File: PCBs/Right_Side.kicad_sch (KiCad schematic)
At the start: 76 parts, among them J4 USB_C_Receptacle, J6 USB_C_Receptacle, U5 W25Q128JVS, U6 XC6206-3.3_SOT, U7 USBLC6-2SC6, U8 RP2040, Y2 Crystal_GND24

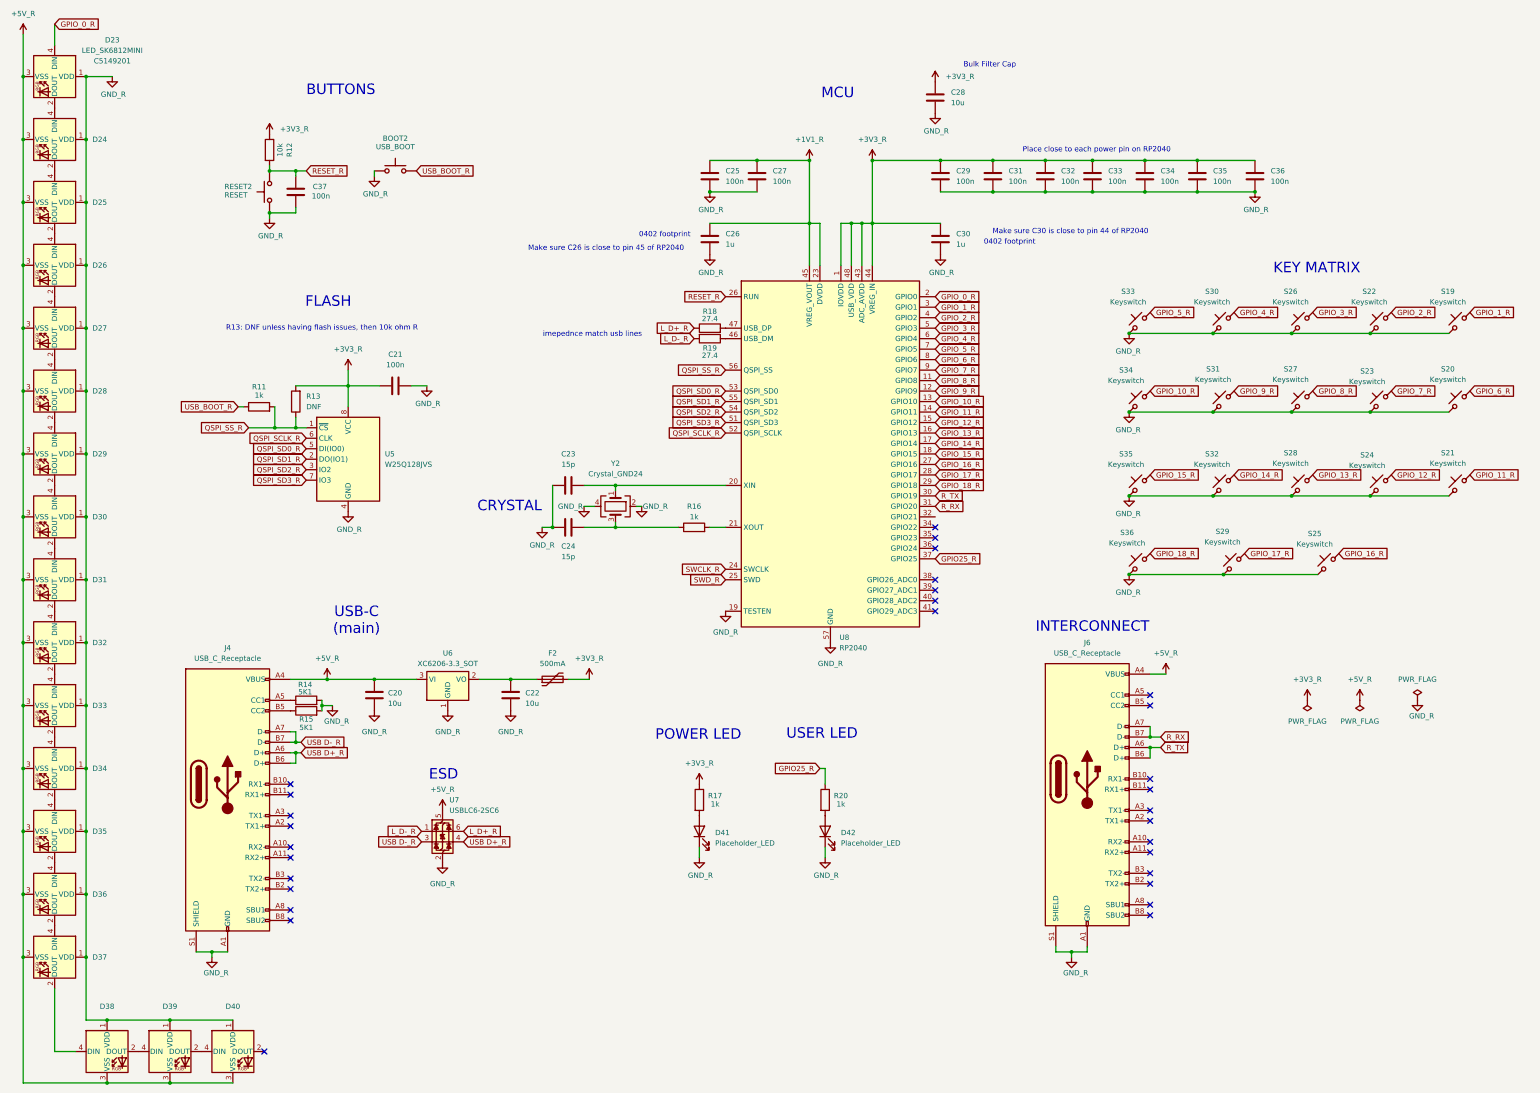
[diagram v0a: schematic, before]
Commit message: mid way right side
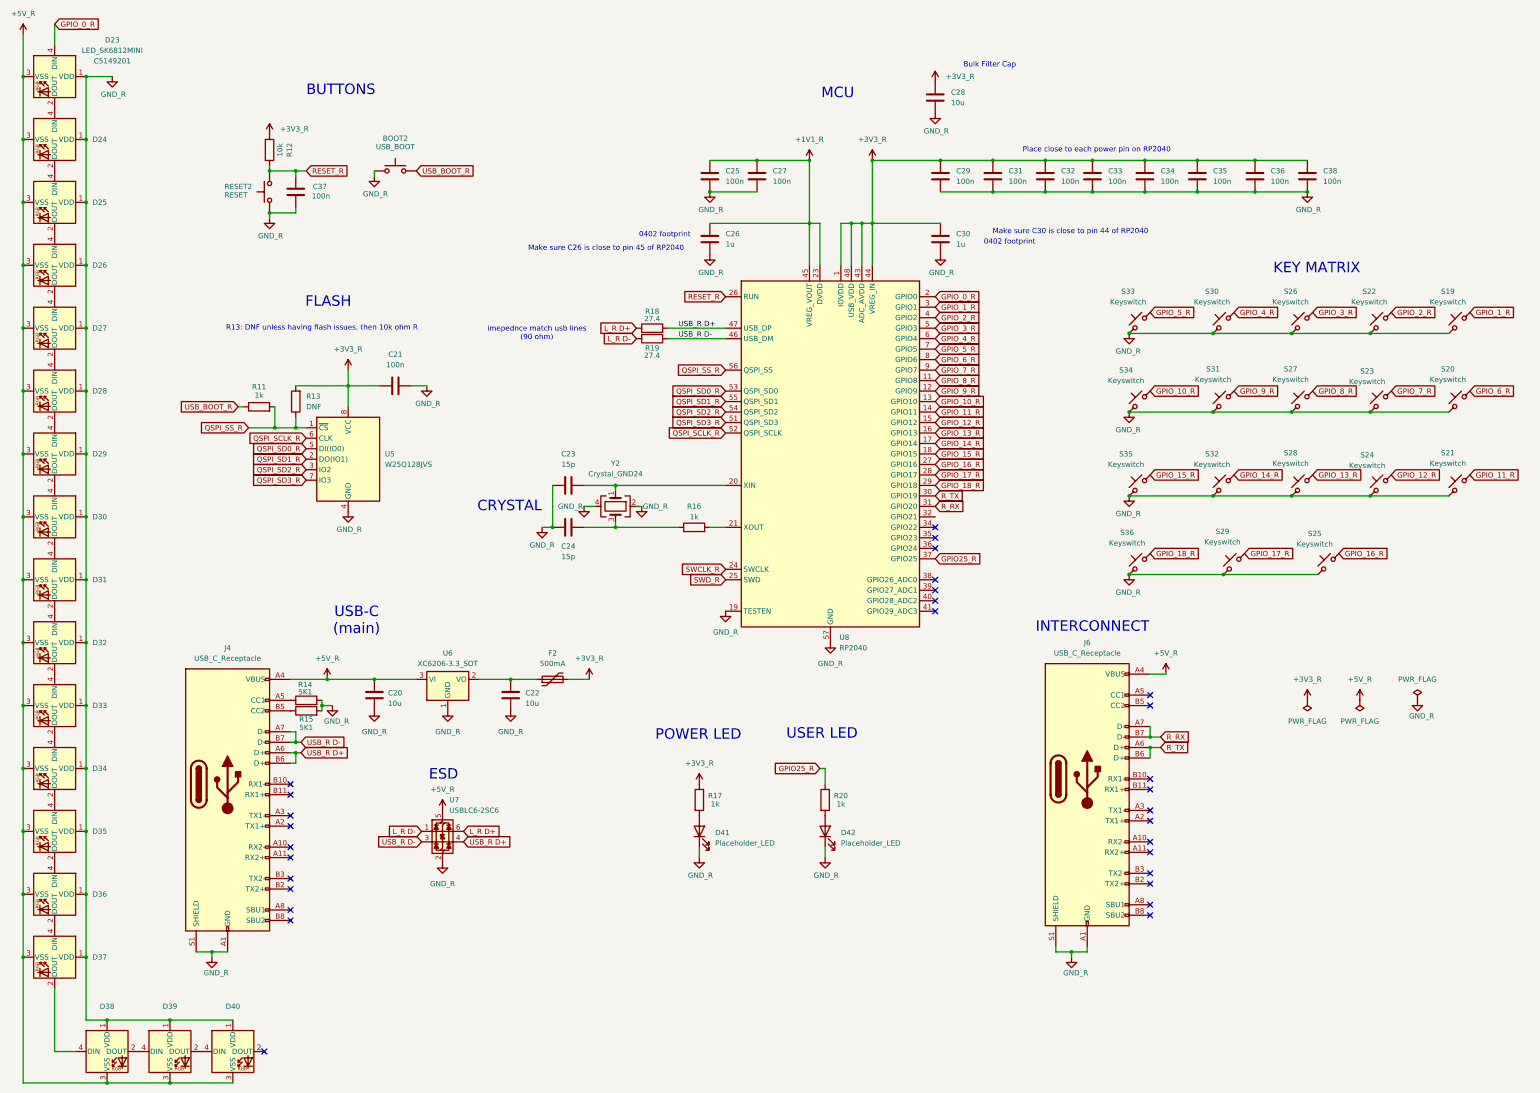
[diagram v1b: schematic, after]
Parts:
- added C38: 100n, Capacitor_SMD:C_0603_1608Metric, symbol Device:C
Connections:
- net USB D+_R is gone; now on net USB_R D+: J4.A6 (D+), J4.B6 (D+), U7.4 (I/O2)
- net USB D-_R is gone; now on net USB_R D-: J4.A7 (D-), J4.B7 (D-), U7.3 (I/O2)
- net +3V3_R: now also C38.1
- net GND_R: now also C38.2
- net USB_R D-: now reaches R19.1, U8.46 (USB_DM)
- net USB_R D+: now reaches R18.2, U8.47 (USB_DP)
- net L_D+_R renamed L_R D+
- net L_D-_R renamed L_R D-
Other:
- note added: "imepednce match usb lines (90 ohm)"
- note removed: "imepednce match usb lines"
- moved on the sheet: R18, R19
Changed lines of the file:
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@@
 	)
 	(junction
+		(at 322.58 54.61)
+		(diameter 0)
+		(color 0 0 0 0)
+	)
+	(junction
+		(at 335.28 62.23)
+		(diameter 0)
+		(color 0 0 0 0)
+	)
+	(junction
 		(at 292.1 115.57)
 		(diameter 0)
@@
 	(wire
 		(pts
+			(xy 180.34 95.25) (xy 194.31 95.25)
+		)
+		(stroke
+			(width 0)
+			(type default)
+		)
+	)
+	(wire
+		(pts
 			(xy 331.47 135.89) (xy 312.42 135.89)
 		)
@@
 	(wire
 		(pts
-			(xy 229.87 69.85) (xy 229.87 80.01)
+			(xy 335.28 62.23) (xy 322.58 62.23)
 		)
 		(stroke
@@
 	(wire
 		(pts
-			(xy 90.17 109.22) (xy 102.87 109.22)
+			(xy 229.87 69.85) (xy 229.87 80.01)
 		)
 		(stroke
@@
 	(wire
 		(pts
-			(xy 24.13 80.01) (xy 24.13 95.25)
+			(xy 90.17 109.22) (xy 102.87 109.22)
 		)
 		(stroke
@@
 	(wire
 		(pts
-			(xy 85.09 119.38) (xy 90.17 119.38)
+			(xy 24.13 80.01) (xy 24.13 95.25)
 		)
 		(stroke
@@
 	(wire
 		(pts
-			(xy 322.58 54.61) (xy 308.61 54.61)
+			(xy 85.09 119.38) (xy 90.17 119.38)
 		)
 		(stroke
@@
 	(wire
 		(pts
+			(xy 180.34 97.79) (xy 194.31 97.79)
+		)
+		(stroke
+			(width 0)
+			(type default)
+		)
+	)
+	(wire
+		(pts
 			(xy 69.85 246.38) (xy 73.66 246.38)
 		)
@@
 	(wire
 		(pts
+			(xy 308.61 54.61) (xy 322.58 54.61)
+		)
+		(stroke
+			(width 0)
+			(type default)
+		)
+	)
+	(wire
+		(pts
 			(xy 24.13 201.93) (xy 24.13 217.17)
 		)
@@
 	(wire
 		(pts
+			(xy 335.28 54.61) (xy 322.58 54.61)
+		)
+		(stroke
+			(width 0)
+			(type default)
+		)
+	)
+	(wire
+		(pts
 			(xy 312.42 135.89) (xy 292.1 135.89)
 		)
@@
 		)
 	)
-	(text "imepednce match usb lines\n"
+	(text "imepednce match usb lines\n(90 ohm)\n"
 		(exclude_from_sim no)
-		(at 162.052 96.774 0)
+		(at 148.59 96.52 0)
 		(effects
 			(font
@@
 		)
 	)
-	(global_label "USB D-_R"
+	(label "USB_R D+"
+		(at 182.88 95.25 0)
+		(effects
+			(font
+				(size 1.27 1.27)
+			)
+			(justify left bottom)
+		)
+	)
+	(label "USB_R D-"
+		(at 182.88 97.79 0)
+		(effects
+			(font
+				(size 1.27 1.27)
+			)
+			(justify left bottom)
+		)
+	)
+	(global_label "USB_R D-"
 		(shape input)
 		(at 120.65 219.71 180)
@@
 		)
 	)
-	(global_label "L_D+_R"
+	(global_label "L_R D+"
 		(shape input)
-		(at 186.69 95.25 180)
+		(at 172.72 95.25 180)
 		(fields_autoplaced yes)
 		(effects
@@
 		)
 		(property "Intersheetrefs" "${INTERSHEET_REFS}"
-			(at 176.6291 95.25 0)
+			(at 162.6591 95.25 0)
 			(effects
 				(font
@@
 		)
 	)
-	(global_label "L_D-_R"
+	(global_label "L_R D-"
 		(shape input)
 		(at 120.65 217.17 180)
@@
 		)
 	)
-	(global_label "L_D+_R"
+	(global_label "L_R D+"
 		(shape input)
 		(at 130.81 217.17 0)
@@
 		)
 	)
-	(global_label "L_D-_R"
+	(global_label "L_R D-"
 		(shape input)
-		(at 186.69 97.79 180)
+		(at 172.72 97.79 180)
 		(fields_autoplaced yes)
 		(effects
@@
 		)
 		(property "Intersheetrefs" "${INTERSHEET_REFS}"
-			(at 176.6291 97.79 0)
+			(at 162.6591 97.79 0)
 			(effects
 				(font
@@
 		)
 	)
-	(global_label "USB D-_R"
+	(global_label "USB_R D-"
 		(shape input)
 		(at 91.44 195.58 0)
@@
 		)
 	)
-	(global_label "USB D+_R"
+	(global_label "USB_R D+"
 		(shape input)
 		(at 130.81 219.71 0)
@@
 		)
 	)
-	(global_label "USB D+_R"
+	(global_label "USB_R D+"
 		(shape input)
 		(at 91.44 198.12 0)
@@
 	(symbol
 		(lib_id "Device:R")
-		(at 190.5 97.79 270)
+		(at 176.53 97.79 270)
 		(unit 1)
 		(exclude_from_sim no)
@@
 		(dnp no)
 		(property "Reference" "R19"
-			(at 190.5 100.076 90)
+			(at 176.53 100.076 90)
 			(effects
 				(font
@@
 		)
 		(property "Value" "27.4"
-			(at 190.5 101.854 90)
+			(at 176.53 101.854 90)
 			(effects
 				(font
@@
 		)
 		(property "Footprint" "Resistor_SMD:R_0603_1608Metric"
-			(at 190.5 96.012 90)
+			(at 176.53 96.012 90)
 			(effects
 				(font
@@
 		)
 		(property "Datasheet" "~"
-			(at 190.5 97.79 0)
+			(at 176.53 97.79 0)
 			(effects
 				(font
@@
 		)
 		(property "Description" "Resistor"
-			(at 190.5 97.79 0)
+			(at 176.53 97.79 0)
 			(effects
 				(font
@@
 	)
 	(symbol
+		(lib_id "Device:C")
+		(at 335.28 58.42 0)
+		(unit 1)
+		(exclude_from_sim no)
+		(in_bom yes)
+		(on_board yes)
+		(dnp no)
+		(fields_autoplaced yes)
+		(property "Reference" "C38"
+			(at 339.09 57.1499 0)
+			(effects
+				(font
+					(size 1.27 1.27)
+				)
+				(justify left)
+			)
+		)
+		(property "Value" "100n"
+			(at 339.09 59.6899 0)
+			(effects
+				(font
+					(size 1.27 1.27)
+				)
+				(justify left)
+			)
+		)
+		(property "Footprint" "Capacitor_SMD:C_0603_1608Metric"
+			(at 336.2452 62.23 0)
+			(effects
+				(font
+					(size 1.27 1.27)
+				)
+				(hide yes)
+			)
+		)
+		(property "Datasheet" "~"
+			(at 335.28 58.42 0)
+			(effects
+				(font
+					(size 1.27 1.27)
+				)
+				(hide yes)
+			)
+		)
+		(property "Description" "Unpolarized capacitor"
+			(at 335.28 58.42 0)
+			(effects
+				(font
+					(size 1.27 1.27)
+				)
+				(hide yes)
+			)
+		)
+		(pin "1"
+		)
+		(pin "2"
+		)
+		(instances
+			(project "CustomKB2040"
+				(path "/1dc59942-63a2-41f5-a9fb-7502b7672a2f/509c21e9-3c87-4ca7-a30c-cd35896bf815"
+					(reference "C38")
+					(unit 1)
+				)
+			)
+		)
+	)
+	(symbol
 		(lib_id "ScottoKeebs:LED_SK6812MINI")
 		(at 31.75 110.49 270)
@@
 	(symbol
 		(lib_id "power:GND")
-		(at 322.58 62.23 0)
+		(at 335.28 62.23 0)
 		(unit 1)
 		(exclude_from_sim no)
@@
 		(dnp no)
 		(property "Reference" "#PWR075"
-			(at 322.58 68.58 0)
+			(at 335.28 68.58 0)
 			(effects
 				(font
@@
 		)
 		(property "Value" "GND_R"
-			(at 322.834 66.548 0)
+			(at 335.534 66.548 0)
 			(effects
 				(font
@@
 		)
 		(property "Footprint" ""
-			(at 322.58 62.23 0)
+			(at 335.28 62.23 0)
 			(effects
 				(font
@@
 		)
 		(property "Datasheet" ""
-			(at 322.58 62.23 0)
+			(at 335.28 62.23 0)
 			(effects
 				(font
@@
 		)
 		(property "Description" "Power symbol creates a global label with name \"GND\" , ground"
-			(at 322.58 62.23 0)
+			(at 335.28 62.23 0)
 			(effects
 				(font
@@
 	(symbol
 		(lib_id "Device:R")
-		(at 190.5 95.25 90)
+		(at 176.53 95.25 90)
 		(unit 1)
 		(exclude_from_sim no)
@@
 		(dnp no)
 		(property "Reference" "R18"
-			(at 190.5 91.186 90)
+			(at 176.53 91.186 90)
 			(effects
 				(font
@@
 		)
 		(property "Value" "27.4"
-			(at 190.5 92.964 90)
+			(at 176.53 92.964 90)
 			(effects
 				(font
@@
 		)
 		(property "Footprint" "Resistor_SMD:R_0603_1608Metric"
-			(at 190.5 97.028 90)
+			(at 176.53 97.028 90)
 			(effects
 				(font
@@
 		)
 		(property "Datasheet" "~"
-			(at 190.5 95.25 0)
+			(at 176.53 95.25 0)
 			(effects
 				(font
@@
 		)
 		(property "Description" "Resistor"
-			(at 190.5 95.25 0)
+			(at 176.53 95.25 0)
 			(effects
 				(font

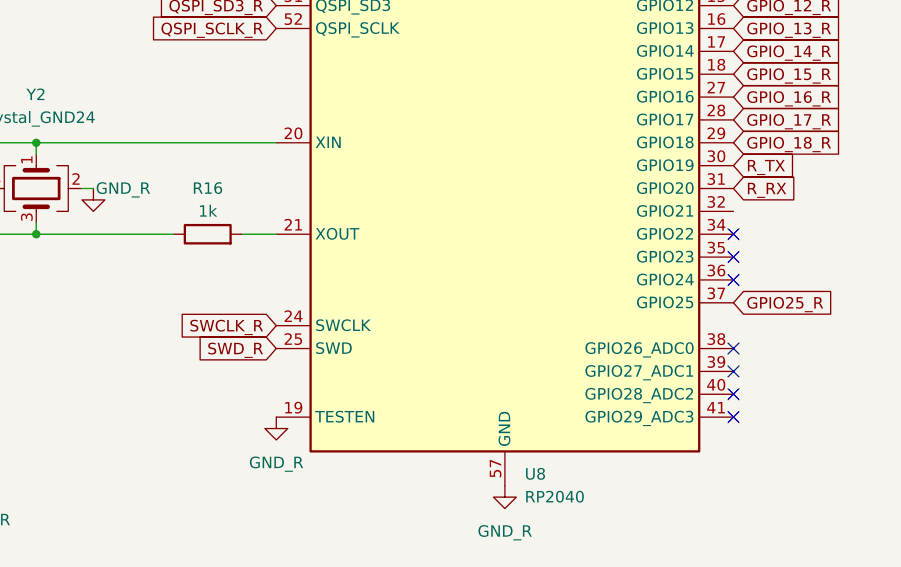
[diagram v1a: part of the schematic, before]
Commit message: making progress
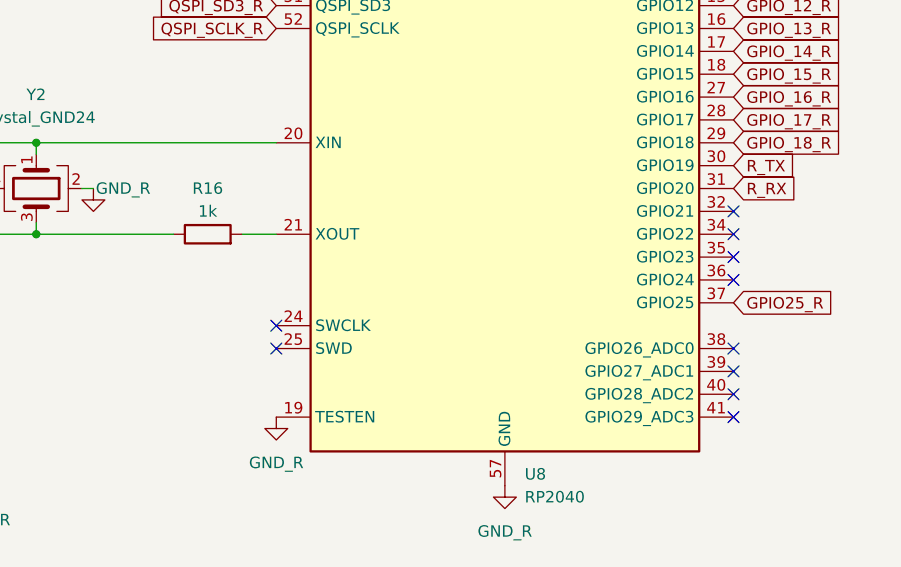
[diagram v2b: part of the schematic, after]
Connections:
- net SWCLK_R: no longer names the net of U8.24 (SWCLK)
- net SWD_R: no longer names the net of U8.25 (SWD)
- no-connect marks 30 -> 33
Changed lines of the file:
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@@
+	)
+	(no_connect
+		(at 194.31 156.21)
 	)
 	(no_connect
@@
 	)
 	(no_connect
+		(at 245.11 140.97)
+	)
+	(no_connect
 		(at 88.9 223.52)
 	)
@@
 	(no_connect
 		(at 88.9 231.14)
+	)
+	(no_connect
+		(at 194.31 153.67)
 	)
 	(no_connect
@@
 		)
 	)
-	(global_label "SWD_R"
-		(shape input)
-		(at 194.31 156.21 180)
+	(global_label "QSPI_SD1_R"
+		(shape input)
+		(at 194.31 113.03 180)
 		(fields_autoplaced yes)
 		(effects
@@
 		)
 		(property "Intersheetrefs" "${INTERSHEET_REFS}"
-			(at 185.1563 156.21 0)
+			(at 180.0158 113.03 0)
 			(effects
 				(font
@@
 		)
 	)
-	(global_label "QSPI_SD1_R"
-		(shape input)
-		(at 194.31 113.03 180)
+	(global_label "GPIO_4_R"
+		(shape input)
+		(at 317.5 91.44 0)
+		(fields_autoplaced yes)
+		(effects
+			(font
+				(size 1.27 1.27)
+			)
+			(justify left)
+		)
+		(property "Intersheetrefs" "${INTERSHEET_REFS}"
+			(at 329.3752 91.44 0)
+			(effects
+				(font
+					(size 1.27 1.27)
+				)
+				(justify left)
+				(hide yes)
+			)
+		)
+	)
+	(global_label "QSPI_SD2_R"
+		(shape input)
+		(at 92.71 129.54 180)
 		(fields_autoplaced yes)
 		(effects
@@
 		)
 		(property "Intersheetrefs" "${INTERSHEET_REFS}"
-			(at 180.0158 113.03 0)
+			(at 78.4158 129.54 0)
 			(effects
 				(font
@@
 		)
 	)
-	(global_label "GPIO_4_R"
-		(shape input)
-		(at 317.5 91.44 0)
-		(fields_autoplaced yes)
-		(effects
-			(font
-				(size 1.27 1.27)
-			)
-			(justify left)
-		)
-		(property "Intersheetrefs" "${INTERSHEET_REFS}"
-			(at 329.3752 91.44 0)
-			(effects
-				(font
-					(size 1.27 1.27)
-				)
-				(justify left)
-				(hide yes)
-			)
-		)
-	)
-	(global_label "QSPI_SD2_R"
-		(shape input)
-		(at 92.71 129.54 180)
-		(fields_autoplaced yes)
-		(effects
-			(font
-				(size 1.27 1.27)
-			)
-			(justify right)
-		)
-		(property "Intersheetrefs" "${INTERSHEET_REFS}"
-			(at 78.4158 129.54 0)
-			(effects
-				(font
-					(size 1.27 1.27)
-				)
-				(justify right)
-				(hide yes)
-			)
-		)
-	)
 	(global_label "USB_R D+"
 		(shape input)
@@
 				(hide yes)
 			)
-		)
-	)
-	(global_label "SWCLK_R"
-		(shape input)
-		(at 194.31 153.67 180)
-		(fields_autoplaced yes)
-		(effects
-			(font
-				(size 1.27 1.27)
-			)
-			(justify right)
-		)
-		(property "Intersheetrefs" "${INTERSHEET_REFS}"
-			(at 182.8582 153.67 0)
-			(effects
-				(font
-					(size 1.27 1.27)
-				)
-				(justify right)
-				(hide yes)
-			)
